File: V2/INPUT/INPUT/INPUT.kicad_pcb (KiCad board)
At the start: 2 copper layers, 80 x 25 mm, 13 parts, among them J1 Conn_01x03, J2 USB_C_Receptacle_USB2.0_16P, J3 Conn_01x03, J4 Conn_01x03, J5 Conn_01x03, J6 Conn_01x03, J7 Conn_01x03, J8 Conn_01x03, J9 Conn_01x03, U1 USBLC6-2P6

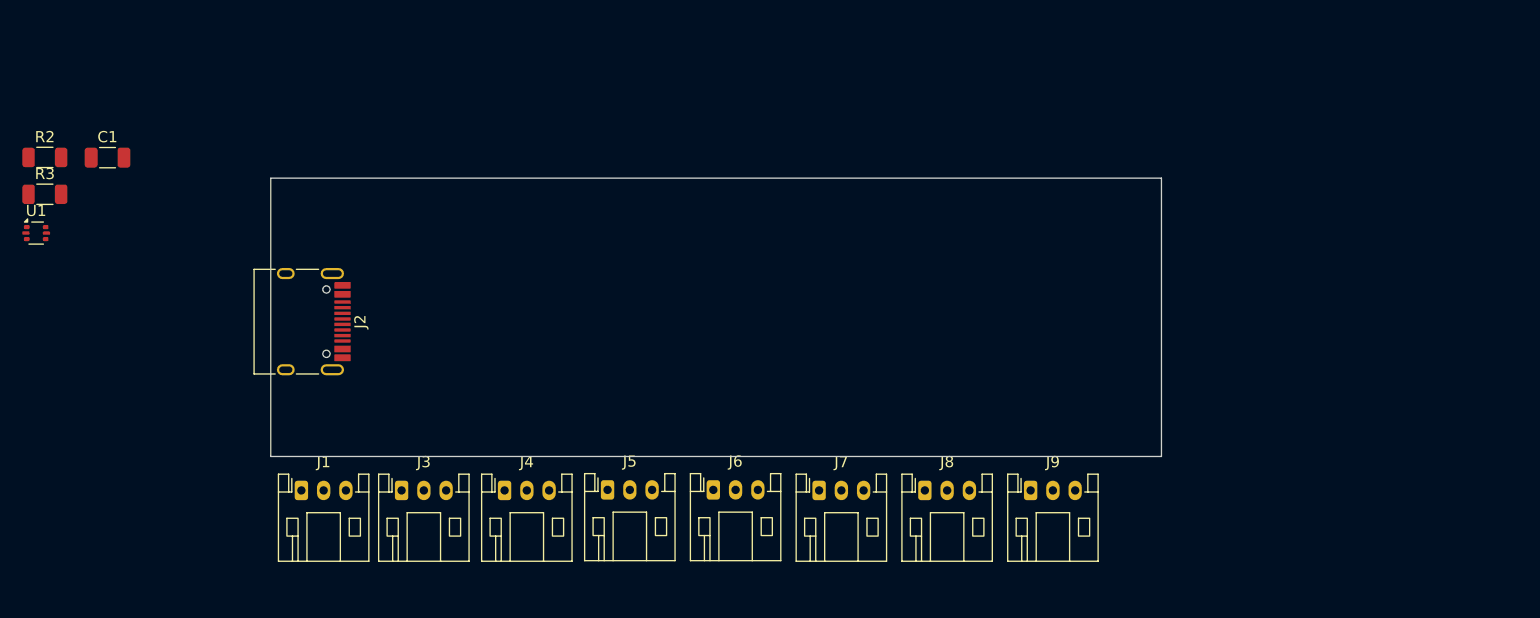
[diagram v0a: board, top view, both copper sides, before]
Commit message: Auto-update: 17.02.2026  0:08:41,99
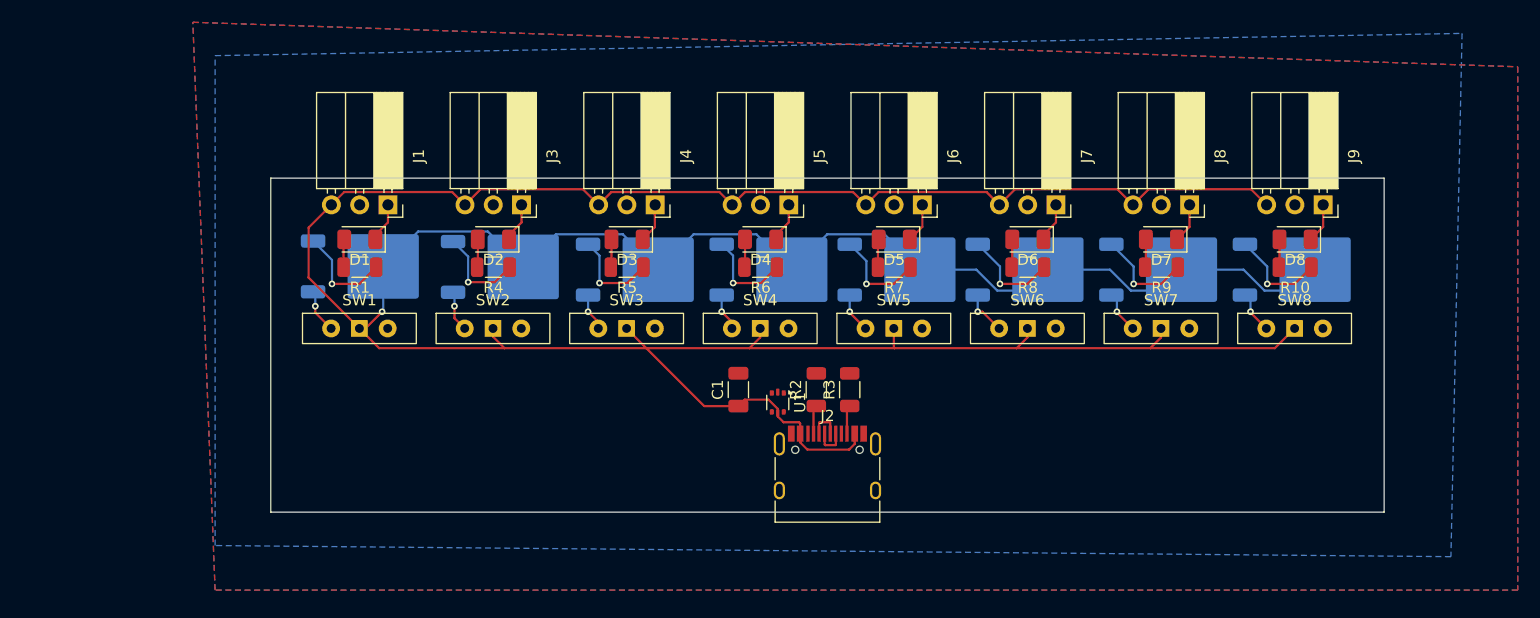
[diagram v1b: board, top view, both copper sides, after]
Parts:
- added D1: LED, LED_SMD:LED_1206_3216Metric, F.Cu at (8.00, 5.50)
- added D2: LED, LED_SMD:LED_1206_3216Metric, F.Cu at (20.0, 5.50)
- added D3: LED, LED_SMD:LED_1206_3216Metric, F.Cu at (32.0, 5.50)
- added D4: LED, LED_SMD:LED_1206_3216Metric, F.Cu at (44.0, 5.50)
- added D5: LED, LED_SMD:LED_1206_3216Metric, F.Cu at (56.0, 5.50)
- added D6: LED, LED_SMD:LED_1206_3216Metric, F.Cu at (68.0, 5.50)
- added D7: LED, LED_SMD:LED_1206_3216Metric, F.Cu at (80.0, 5.50)
- added D8: LED, LED_SMD:LED_1206_3216Metric, F.Cu at (92.0, 5.50)
- added Q1: QM6006D, Package_TO_SOT_SMD:TO-252-2, B.Cu at (21.4, 7.97)
- added Q2: QM6006D, Package_TO_SOT_SMD:TO-252-2, B.Cu at (8.84, 7.93)
- added Q3: QM6006D, Package_TO_SOT_SMD:TO-252-2, B.Cu at (33.5, 8.22)
- added Q4: QM6006D, Package_TO_SOT_SMD:TO-252-2, B.Cu at (45.5, 8.22)
- added Q5: QM6006D, Package_TO_SOT_SMD:TO-252-2, B.Cu at (57.0, 8.22)
- added Q6: QM6006D, Package_TO_SOT_SMD:TO-252-2, B.Cu at (68.5, 8.22)
- added Q7: QM6006D, Package_TO_SOT_SMD:TO-252-2, B.Cu at (80.5, 8.22)
- added Q8: QM6006D, Package_TO_SOT_SMD:TO-252-2, B.Cu at (92.5, 8.22)
- added R1: R, Resistor_SMD:R_1206_3216Metric, F.Cu at (8.00, 8.00)
- added R10: R, Resistor_SMD:R_1206_3216Metric, F.Cu at (92.0, 8.00)
- added R4: R, Resistor_SMD:R_1206_3216Metric, F.Cu at (20.0, 8.00)
- added R5: R, Resistor_SMD:R_1206_3216Metric, F.Cu at (32.0, 8.00)
- added R6: R, Resistor_SMD:R_1206_3216Metric, F.Cu at (44.0, 8.00)
- added R7: R, Resistor_SMD:R_1206_3216Metric, F.Cu at (56.0, 8.00)
- added R8: R, Resistor_SMD:R_1206_3216Metric, F.Cu at (68.0, 8.00)
- added R9: R, Resistor_SMD:R_1206_3216Metric, F.Cu at (80.0, 8.00)
- added SW1: SW_SPST, Button_Switch_THT:SW_Slide-03_Wuerth-WS-SLTV_10x2.5x6.4_P2.54mm, F.Cu at (7.96, 13.5)
- added SW2: SW_SPST, Button_Switch_THT:SW_Slide-03_Wuerth-WS-SLTV_10x2.5x6.4_P2.54mm, F.Cu at (20.0, 13.5)
- added SW3: SW_SPST, Button_Switch_THT:SW_Slide-03_Wuerth-WS-SLTV_10x2.5x6.4_P2.54mm, F.Cu at (32.0, 13.5)
- added SW4: SW_SPST, Button_Switch_THT:SW_Slide-03_Wuerth-WS-SLTV_10x2.5x6.4_P2.54mm, F.Cu at (44.0, 13.5)
- added SW5: SW_SPST, Button_Switch_THT:SW_Slide-03_Wuerth-WS-SLTV_10x2.5x6.4_P2.54mm, F.Cu at (56.0, 13.5)
- added SW6: SW_SPST, Button_Switch_THT:SW_Slide-03_Wuerth-WS-SLTV_10x2.5x6.4_P2.54mm, F.Cu at (68.0, 13.5)
- added SW7: SW_SPST, Button_Switch_THT:SW_Slide-03_Wuerth-WS-SLTV_10x2.5x6.4_P2.54mm, F.Cu at (80.0, 13.5)
- added SW8: SW_SPST, Button_Switch_THT:SW_Slide-03_Wuerth-WS-SLTV_10x2.5x6.4_P2.54mm, F.Cu at (92.0, 13.5)
- J1, J3, J4, J5, J6, J7, J8, J9: footprint Connector_JST:JST_PH_S3B-PH-K_1x03_P2.00mm_Horizontal -> Connector_PinSocket_2.54mm:PinSocket_1x03_P2.54mm_Horizontal
- moved R3 74.4 mm to (52.0, 19.0), turned to 90 degrees
- moved R2 72.4 mm to (49.0, 19.0), turned to 90 degrees
- moved U1 68.3 mm to (45.5, 20.1), turned to -90 degrees
- moved C1 60.4 mm to (42.0, 19.0), turned to 90 degrees
- moved J2 49.6 mm to (50.0, 27.0), turned to 0 degrees
- moved J9 36.7 mm to (94.5, 2.40), turned to -90 degrees
- moved J8 35.0 mm to (82.5, 2.40), turned to -90 degrees
- moved J7 33.3 mm to (70.5, 2.40), turned to -90 degrees
- moved J6 31.7 mm to (58.5, 2.40), turned to -90 degrees
- moved J5 30.3 mm to (46.5, 2.40), turned to -90 degrees
- moved J4 29.0 mm to (34.5, 2.40), turned to -90 degrees
- moved J3 27.8 mm to (22.5, 2.40), turned to -90 degrees
- moved J1 26.8 mm to (10.5, 2.40), turned to -90 degrees
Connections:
- J1 pad 1: +5V -> Net-(D1-K)
- J1 pad 3: GND -> +5V
- J3 pad 1: +5V -> Net-(D2-K)
- J3 pad 3: GND -> +5V
- J4 pad 1: +5V -> Net-(D3-K)
- J4 pad 3: GND -> +5V
- J5 pad 1: +5V -> Net-(D4-K)
- J5 pad 3: GND -> +5V
- J6 pad 1: +5V -> Net-(D5-K)
- J6 pad 3: GND -> +5V
- J7 pad 1: +5V -> Net-(D6-K)
- J7 pad 3: GND -> +5V
- J8 pad 1: +5V -> Net-(D7-K)
- J8 pad 3: GND -> +5V
- J9 pad 1: +5V -> Net-(D8-K)
- J9 pad 3: GND -> +5V
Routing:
- net +5V: track 0.00 -> 334.7 mm, vias 0 -> 1
- net Net-(Q2-S): track 0.00 -> 9.23 mm, vias 0 -> 1
- net Net-(Q8-S): track 0.00 -> 8.97 mm, vias 0 -> 1
- net Net-(Q7-S): track 0.00 -> 8.97 mm, vias 0 -> 1
- net Net-(Q6-S): track 0.00 -> 8.97 mm, vias 0 -> 1
- net Net-(Q5-S): track 0.00 -> 8.77 mm, vias 0 -> 1
- net Net-(Q1-S): track 0.00 -> 8.50 mm, vias 0 -> 1
- net Net-(Q4-S): track 0.00 -> 8.43 mm, vias 0 -> 1
- net Net-(Q3-S): track 0.00 -> 8.43 mm, vias 0 -> 1
- net Net-(Q6-G): track 0.00 -> 4.04 mm, vias 0 -> 1
- net Net-(Q2-G): track 0.00 -> 3.96 mm, vias 0 -> 1
- net Net-(Q8-G): track 0.00 -> 3.80 mm, vias 0 -> 1
- net Net-(Q7-G): track 0.00 -> 3.80 mm, vias 0 -> 1
- net Net-(Q1-G): track 0.00 -> 3.68 mm, vias 0 -> 1
- net Net-(D8-K): track 0.00 -> 3.65 mm
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- added copper zone on B.Cu, net (none)
- added copper zone on B.Cu, net GND
- added copper zone on F.Cu, net GND
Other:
- board size 80 x 25 mm -> 100 x 30 mm

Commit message: Auto-update: 26.02.2026  0:22:57,46
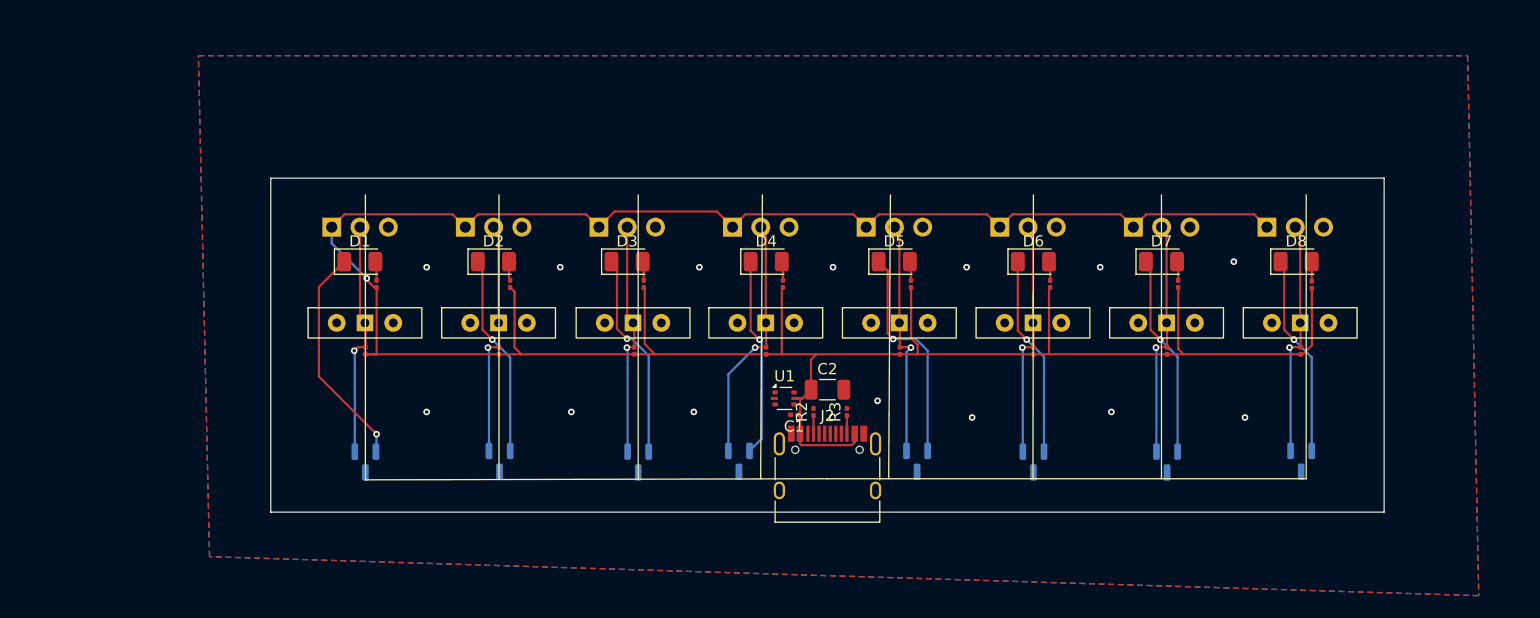
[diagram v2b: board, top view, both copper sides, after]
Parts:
- added C2: 10µF, Capacitor_SMD:C_1206_3216Metric, F.Cu at (50.0, 19.0)
- added R11: 10k, Resistor_SMD:R_0201_0603Metric, F.Cu at (56.5, 15.5)
- added R12: R, Resistor_SMD:R_0201_0603Metric, F.Cu at (57.5, 9.50)
- added R13: 10k, Resistor_SMD:R_0201_0603Metric, F.Cu at (68.5, 15.5)
- added R14: R, Resistor_SMD:R_0201_0603Metric, F.Cu at (70.0, 9.50)
- added R15: 10k, Resistor_SMD:R_0201_0603Metric, F.Cu at (80.5, 15.5)
- added R16: R, Resistor_SMD:R_0201_0603Metric, F.Cu at (81.5, 9.50)
- added R17: 10k, Resistor_SMD:R_0201_0603Metric, F.Cu at (92.5, 15.5)
- added R18: R, Resistor_SMD:R_0201_0603Metric, F.Cu at (93.5, 9.57)
- C1: footprint Capacitor_SMD:C_1206_3216Metric -> Capacitor_SMD:C_0201_0603Metric
- J1, J3, J4, J5, J6, J7, J8, J9: moved to B.Cu
- Q1, Q2, Q3, Q4, Q5, Q6, Q7, Q8: footprint Package_TO_SOT_SMD:TO-252-2 -> Package_TO_SOT_SMD:SOT-23
- R1, R10, R2, R3, R6, R8: footprint Resistor_SMD:R_1206_3216Metric -> Resistor_SMD:R_0201_0603Metric
- R4, R5, R7, R9: value R -> 10k; footprint Resistor_SMD:R_1206_3216Metric -> Resistor_SMD:R_0201_0603Metric
- moved R10 46.0 mm to (46.0, 9.50), turned to -90 degrees
- moved R9 36.3 mm to (44.5, 15.5), turned to -90 degrees
- moved R8 34.5 mm to (33.5, 9.50), turned to -90 degrees
- moved R7 24.5 mm to (32.7, 15.5), turned to -90 degrees
- moved R6 22.5 mm to (21.5, 9.50), turned to -90 degrees
- moved Q2 17.6 mm to (8.50, 25.5), turned to -90 degrees
- moved Q4 17.6 mm to (42.0, 25.4), turned to -90 degrees
- moved Q1 17.5 mm to (20.6, 25.4), turned to -90 degrees
- moved Q3 17.3 mm to (33.0, 25.5), turned to -90 degrees
- moved Q6 17.3 mm to (68.5, 25.5), turned to -90 degrees
- moved Q7 17.3 mm to (80.5, 25.5), turned to -90 degrees
- moved Q5 17.2 mm to (58.0, 25.4), turned to -90 degrees
- moved Q8 17.2 mm to (92.5, 25.4), turned to -90 degrees
- moved R4 13.7 mm to (8.50, 15.5), turned to -90 degrees
- moved R5 13.7 mm to (20.5, 15.5), turned to -90 degrees
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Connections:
- J1 pad 1: Net-(D1-K) -> +5V
- J1 pad 2: unconnected-(J1-Pin_2-Pad2) -> Net-(J1-Pin_2)
- J1 pad 3: +5V -> GND
- J2 pad S1: unconnected-(J2-SHIELD-PadS1) -> GND
- J3 pad 1: Net-(D2-K) -> +5V
- J3 pad 2: unconnected-(J3-Pin_2-Pad2) -> Net-(J3-Pin_2)
- J3 pad 3: +5V -> GND
- J4 pad 1: Net-(D3-K) -> +5V
- J4 pad 2: unconnected-(J4-Pin_2-Pad2) -> Net-(J4-Pin_2)
- J4 pad 3: +5V -> GND
- J5 pad 1: Net-(D4-K) -> +5V
- J5 pad 2: unconnected-(J5-Pin_2-Pad2) -> Net-(J5-Pin_2)
- J5 pad 3: +5V -> GND
- J6 pad 1: Net-(D5-K) -> +5V
- J6 pad 2: unconnected-(J6-Pin_2-Pad2) -> Net-(J6-Pin_2)
- J6 pad 3: +5V -> GND
- J7 pad 1: Net-(D6-K) -> +5V
- J7 pad 2: unconnected-(J7-Pin_2-Pad2) -> Net-(J7-Pin_2)
- J7 pad 3: +5V -> GND
- J8 pad 1: Net-(D7-K) -> +5V
- J8 pad 2: unconnected-(J8-Pin_2-Pad2) -> Net-(J8-Pin_2)
- J8 pad 3: +5V -> GND
- J9 pad 1: Net-(D8-K) -> +5V
- J9 pad 2: unconnected-(J9-Pin_2-Pad2) -> Net-(J9-Pin_2)
- J9 pad 3: +5V -> GND
- Q1 pad 1: Net-(Q1-G) -> Net-(J3-Pin_2)
- Q1 pad 2: +5V -> Net-(D2-K)
- Q1 pad 3: Net-(Q1-S) -> GND
- Q2 pad 1: Net-(Q2-G) -> Net-(J1-Pin_2)
- Q2 pad 2: +5V -> Net-(D1-K)
- Q2 pad 3: Net-(Q2-S) -> GND
- Q3 pad 1: Net-(Q3-G) -> Net-(J4-Pin_2)
- Q3 pad 2: +5V -> Net-(D3-K)
- Q3 pad 3: Net-(Q3-S) -> GND
- Q4 pad 1: Net-(Q4-G) -> Net-(J5-Pin_2)
- Q4 pad 2: +5V -> Net-(D4-K)
- Q4 pad 3: Net-(Q4-S) -> GND
- Q5 pad 1: Net-(Q5-G) -> Net-(J6-Pin_2)
- Q5 pad 2: +5V -> Net-(D5-K)
- Q5 pad 3: Net-(Q5-S) -> GND
- Q6 pad 1: Net-(Q6-G) -> Net-(J7-Pin_2)
- Q6 pad 2: +5V -> Net-(D6-K)
- Q6 pad 3: Net-(Q6-S) -> GND
- Q7 pad 1: Net-(Q7-G) -> Net-(J8-Pin_2)
- Q7 pad 2: +5V -> Net-(D7-K)
- Q7 pad 3: Net-(Q7-S) -> GND
- Q8 pad 1: Net-(Q8-G) -> Net-(J9-Pin_2)
- Q8 pad 2: +5V -> Net-(D8-K)
- Q8 pad 3: Net-(Q8-S) -> GND
- R1 pad 1: Net-(Q2-S) -> Net-(D1-A)
- R1 pad 2: Net-(D1-A) -> +5V
- R10 pad 1: Net-(Q8-S) -> Net-(D4-A)
- R10 pad 2: Net-(D8-A) -> +5V
- R4 pad 1: Net-(Q1-S) -> Net-(J1-Pin_2)
- R4 pad 2: Net-(D2-A) -> +5V
- R5 pad 1: Net-(Q3-S) -> Net-(J3-Pin_2)
- R5 pad 2: Net-(D3-A) -> +5V
- R6 pad 1: Net-(Q4-S) -> Net-(D2-A)
- R6 pad 2: Net-(D4-A) -> +5V
- R7 pad 1: Net-(Q5-S) -> Net-(J4-Pin_2)
- R7 pad 2: Net-(D5-A) -> +5V
- R8 pad 1: Net-(Q6-S) -> Net-(D3-A)
- R8 pad 2: Net-(D6-A) -> +5V
- R9 pad 1: Net-(Q7-S) -> Net-(J5-Pin_2)
- R9 pad 2: Net-(D7-A) -> +5V
- SW1 pad 1: +5V -> Net-(J1-Pin_2)
- SW1 pad 2: Net-(Q2-G) -> GND
- SW2 pad 1: +5V -> Net-(J3-Pin_2)
- SW2 pad 2: Net-(Q1-G) -> GND
- SW3 pad 1: +5V -> Net-(J4-Pin_2)
- SW3 pad 2: Net-(Q3-G) -> GND
- SW4 pad 1: +5V -> Net-(J5-Pin_2)
- SW4 pad 2: Net-(Q4-G) -> GND
- SW5 pad 1: +5V -> Net-(J6-Pin_2)
- SW5 pad 2: Net-(Q5-G) -> GND
- SW6 pad 1: +5V -> Net-(J7-Pin_2)
- SW6 pad 2: Net-(Q6-G) -> GND
- SW7 pad 1: +5V -> Net-(J8-Pin_2)
- SW7 pad 2: Net-(Q7-G) -> GND
- SW8 pad 1: +5V -> Net-(J9-Pin_2)
- SW8 pad 2: Net-(Q8-G) -> GND
- U1 pad 1: Net-(J2-D--PadA7) -> unconnected-(U1-I/O1-Pad1)
- U1 pad 3: Net-(J2-D+-PadA6) -> unconnected-(U1-I/O2-Pad3)
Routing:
- net +5V: track 334.7 -> 248.9 mm
- net Net-(J5-Pin_2): track 0.00 -> 22.3 mm, vias 0 -> 1
- net Net-(J6-Pin_2): track 0.00 -> 21.4 mm, vias 0 -> 1
- net Net-(J8-Pin_2): track 0.00 -> 21.4 mm, vias 0 -> 1
- net Net-(J7-Pin_2): track 0.00 -> 21.4 mm, vias 0 -> 1
- net Net-(J3-Pin_2): track 0.00 -> 21.3 mm, vias 0 -> 1
- net Net-(J9-Pin_2): track 0.00 -> 21.3 mm, vias 0 -> 1
- net Net-(J1-Pin_2): track 0.00 -> 21.2 mm, vias 0 -> 1
- net Net-(J4-Pin_2): track 0.00 -> 21.1 mm, vias 0 -> 1
- net Net-(D1-K): track 3.57 -> 20.2 mm, vias 0 -> 1
- net Net-(D5-K): track 3.65 -> 20.0 mm, vias 0 -> 1
- net Net-(D3-K): track 3.65 -> 18.7 mm, vias 0 -> 1
- net Net-(D7-K): track 3.65 -> 18.2 mm, vias 0 -> 1
- net Net-(D2-K): track 3.65 -> 18.2 mm, vias 0 -> 1
- net Net-(D8-K): track 3.65 -> 18.2 mm, vias 0 -> 1
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- removed copper zone on B.Cu, net (none)
